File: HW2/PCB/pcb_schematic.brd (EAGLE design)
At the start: 50 x 50 mm, 20 parts, among them J1 USB-MB-H

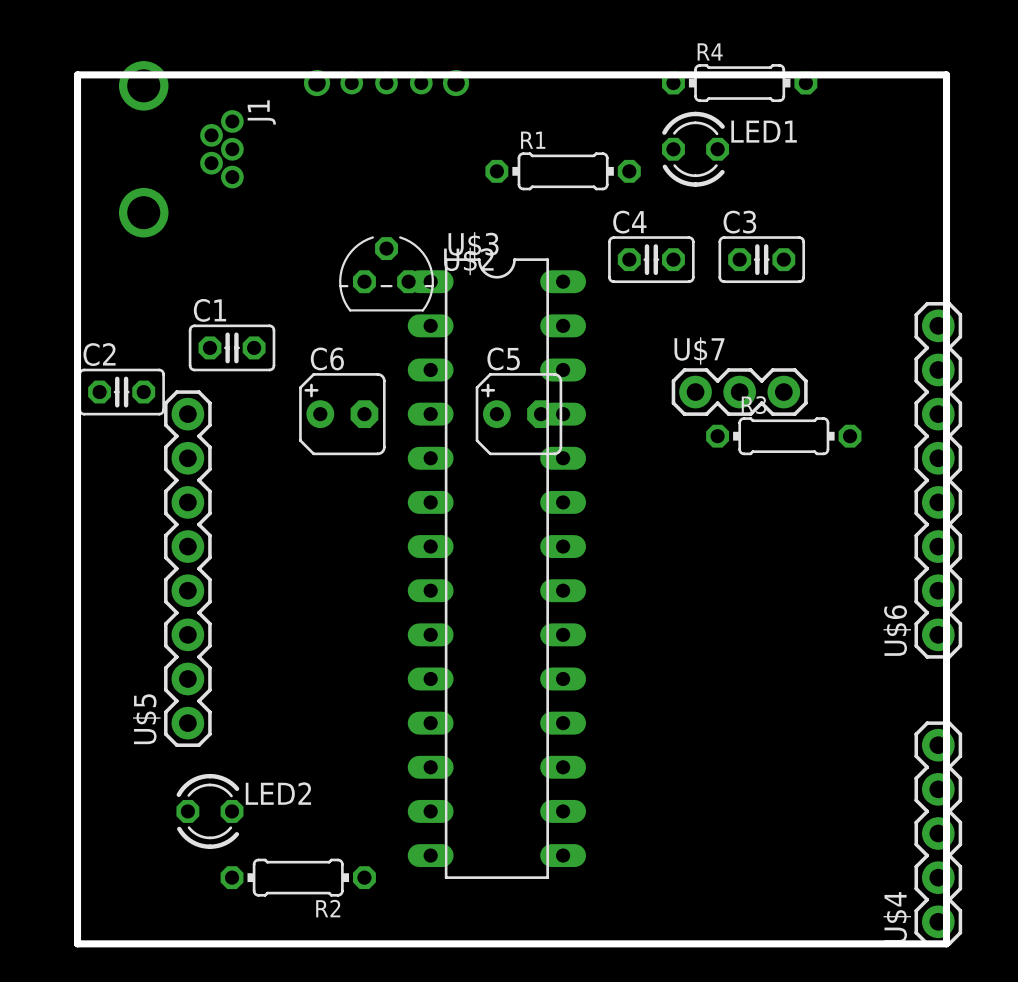
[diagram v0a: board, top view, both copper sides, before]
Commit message: PCB is closer.
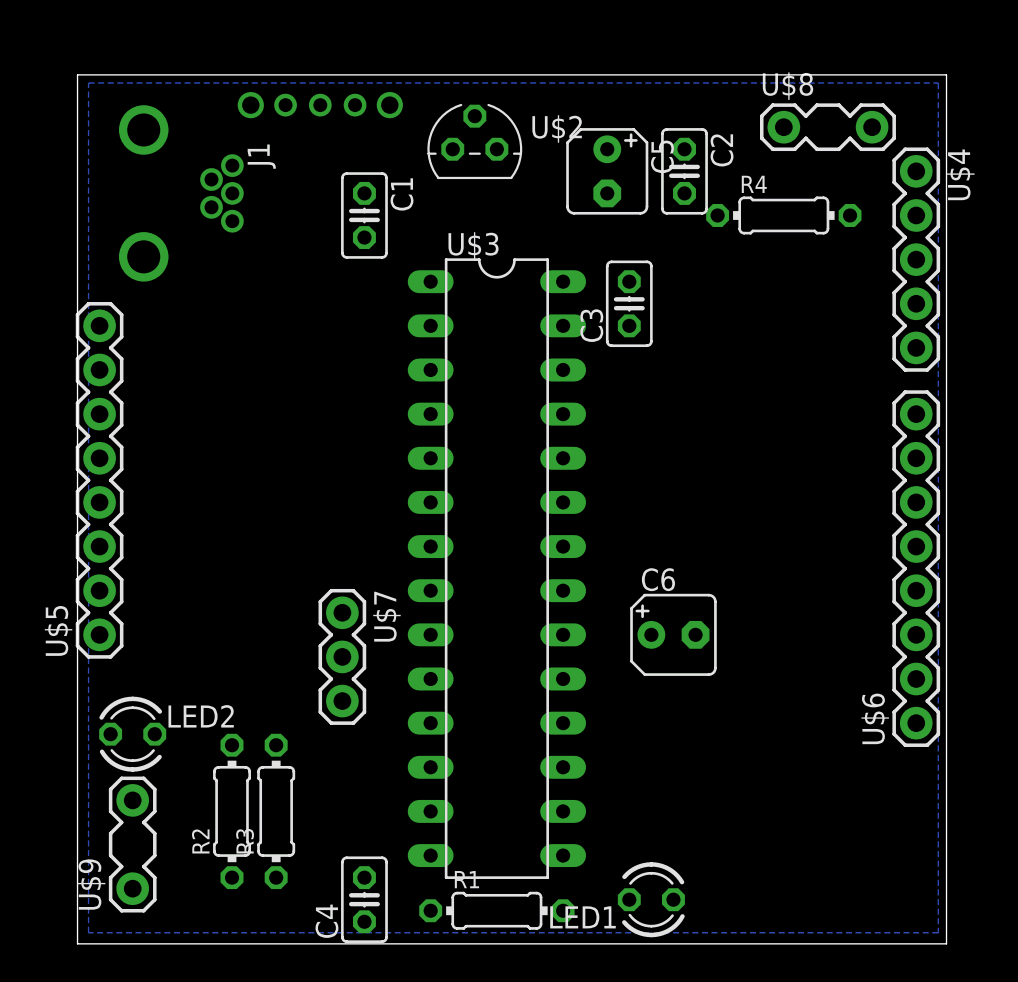
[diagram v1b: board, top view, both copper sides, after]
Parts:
- added U$8, U$9: SWITCH, pcb_library:SWITCH
- moved LED1 43.3 mm to (33.0, 2.54), turned to 180 degrees
- moved U$4 43.2 mm to (48.3, 44.5), turned to 270 degrees
- moved R1 42.7 mm to (24.1, 1.91)
- moved C4 40.4 mm to (16.5, 2.54), turned to 90 degrees
- moved R3 36.3 mm to (11.4, 7.62), turned to 90 degrees
- moved C2 34.8 mm to (34.9, 44.5), turned to 270 degrees
- moved U$7 24.0 mm to (15.2, 19.1), turned to 270 degrees
- moved C6 22.9 mm to (34.3, 17.8)
- moved C5 14.9 mm to (30.5, 44.5), turned to 270 degrees
- moved C1 10.8 mm to (16.5, 41.9), turned to 270 degrees
- moved U$2 9.16 mm to (22.9, 45.7)
- moved R4 8.03 mm to (40.6, 41.9)
- moved C3 8.03 mm to (31.8, 36.8), turned to 90 degrees
- moved U$5 7.18 mm to (1.27, 17.8)
- moved LED2 6.29 mm to (3.17, 12.1)
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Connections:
- net B4/USER: now also U$8.1
- net GND: now also U$8.3, U$9.3
- net MCLR: now also U$9.1
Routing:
- added copper zone on layer 16, net GND
